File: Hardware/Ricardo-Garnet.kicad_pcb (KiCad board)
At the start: 4 copper layers, 38.5 x 90 mm, 193 parts, among them IC3 AP2205-W5-7, IC4 TPS61089RNRR, IC5 ADS131M04IRUKR, J1 RBUS, J2 USB_C_Receptacle_USB2.0, J3 Rotary Pot, J4 Conn_01x02_Male, J5 Conn_01x02_Male, J7 Conn_01x02_Male, J8 Conn_01x02_Male, J9 Conn_01x02_Male, P4 IN+, P5 IN-, P6 MOTOR1, P7 MOTOR2, P9 MOTOR3, Q1 IRFS7530, Q2 IRFS7530, Q3 IRFS7530, Q4 IRFS7530, Q5 IRFS7530, Q6 IRFS7530, U1 ESP32-S3, U10 MAX31856, U11 MAX31856, U3 DRV8302, U4 LM66200DRLR, U5 SC4215, U6 SN65HVD230, U7 MAX77827AEFD+T, U9 THVD2429, Y2 R940000171

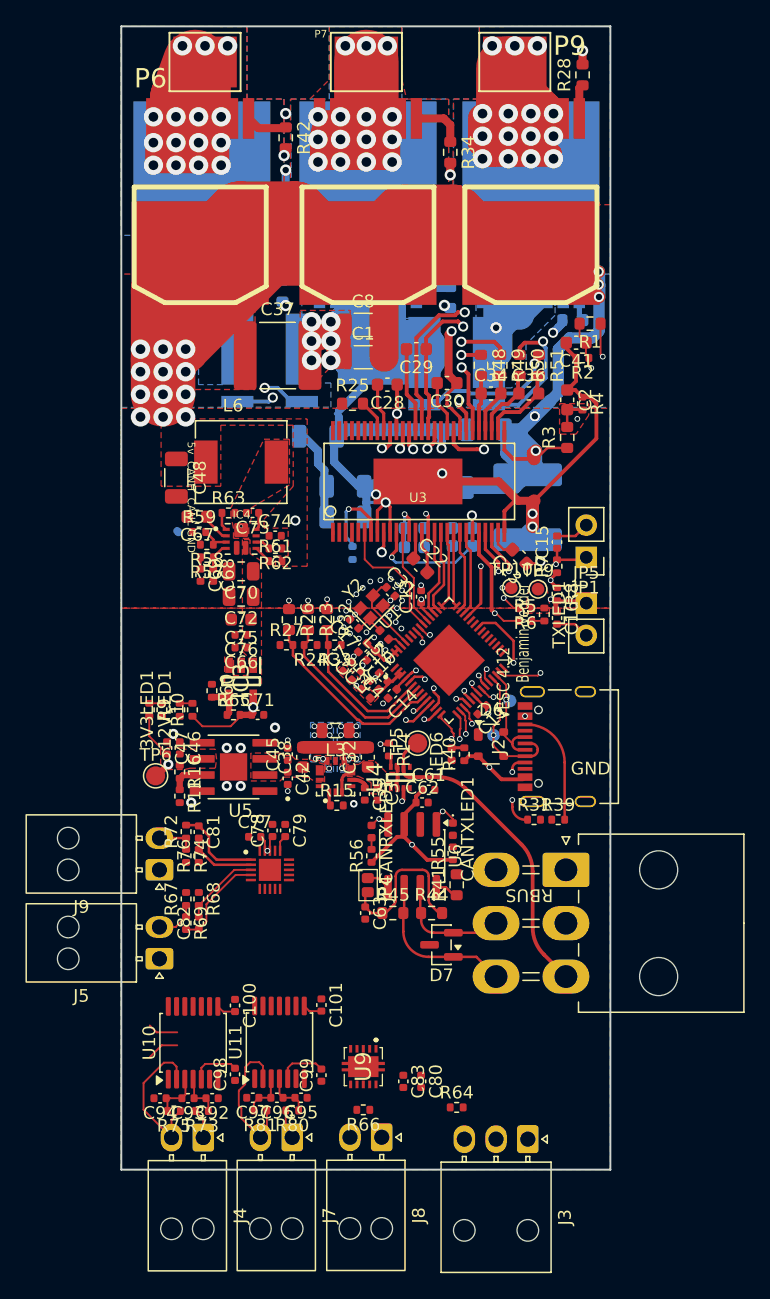
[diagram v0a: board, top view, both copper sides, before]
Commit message: close to 1st done
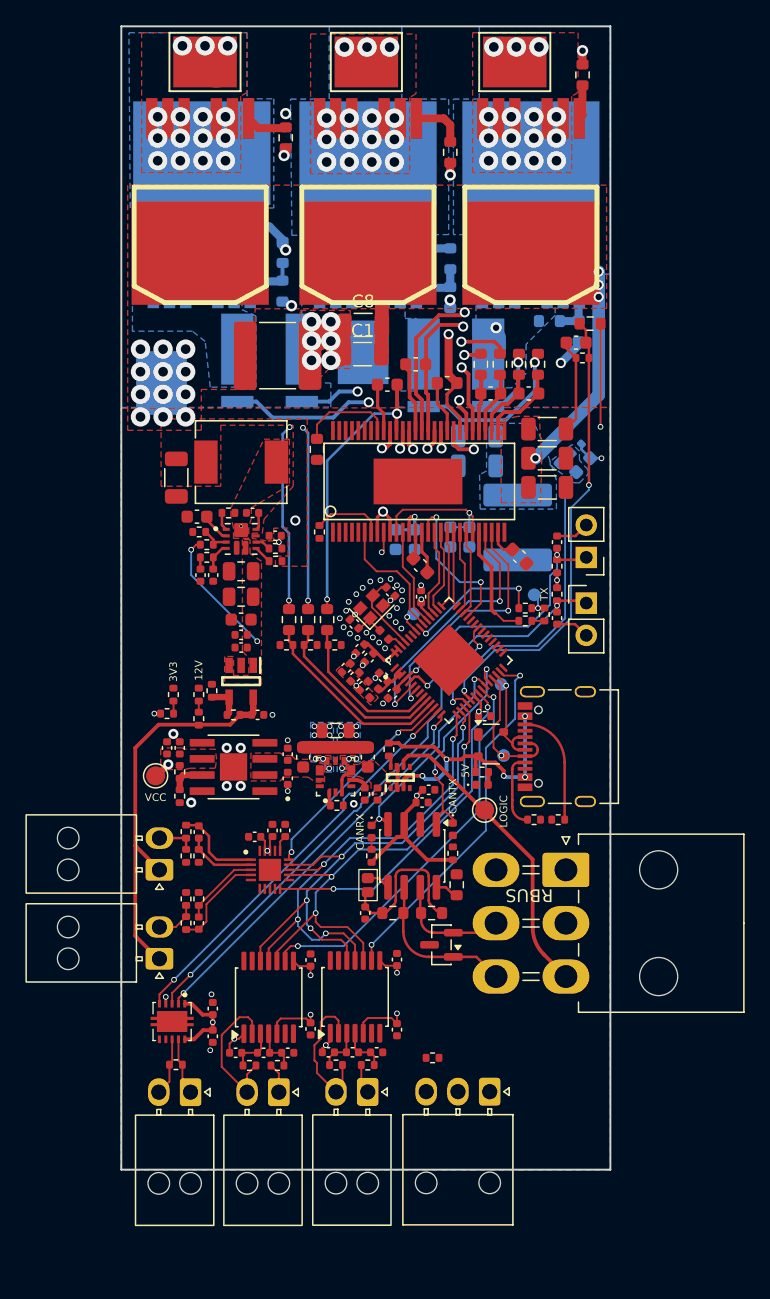
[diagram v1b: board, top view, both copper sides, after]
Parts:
- removed C34, C36: 2.2n, Capacitor_SMD:C_0603_1608Metric
- removed R48, R49, R50, R51: 100R, Resistor_SMD:R_0603_1608Metric
- added C19: 2.2n, Capacitor_SMD:C_0603_1608Metric, F.Cu at (107.6, 108.9)
- added C21: 2.2n, Capacitor_SMD:C_0603_1608Metric, F.Cu at (110.6, 108.9)
- added R12: 100R, Resistor_SMD:R_0603_1608Metric, F.Cu at (106.8, 106.6)
- added R13: 100R, Resistor_SMD:R_0603_1608Metric, F.Cu at (108.3, 106.6)
- added R17: 100R, Resistor_SMD:R_0603_1608Metric, F.Cu at (109.8, 106.6)
- added R18: 100R, Resistor_SMD:R_0603_1608Metric, F.Cu at (111.3, 106.6)
- C2, R3, R4: moved to B.Cu
- C43, C44, C49, R20: moved to F.Cu
- RXD: renamed from TP10; moved to B.Cu
- TXD: renamed from TP9; moved to B.Cu
- moved C43 18.1 mm to (112.0, 111.7)
- moved C80 17.4 mm to (85.7, 157.3)
- moved C49 16.1 mm to (112.0, 116.3)
- moved C44 16.0 mm to (112.0, 114.0)
- moved J8 15.5 mm to (84.0, 163.9)
- moved U9 15.5 mm to (82.5, 158.3)
- moved C83 15.4 mm to (85.7, 159.5)
- moved R66 15.2 mm to (82.8, 161.7)
- moved R30 10.5 mm to (112.2, 103.2), turned to 0 degrees
- moved RXD 7.97 mm to (101.5, 126.2), turned to 180 degrees
- moved LOGIC 7.45 mm to (107.1, 141.7)
- moved C96 6.94 mm to (96.7, 160.8)
- moved C97 6.94 mm to (94.8, 160.8)
- moved C98 6.94 mm to (93.4, 158.9)
- moved C99 6.94 mm to (100.2, 159.0)
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- renumbered 12VLED1 to 12V, 3V3LED1 to 3V3, CANRXLED1 to CANRX, CANTXLED1 to CANTX, TP2 to Dat+, TP1 to Dat-, TP5 to LOGIC, TXLED1 to TX, TP6 to VCC
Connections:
- net /Mosfet driver/H1_VS renamed /Mosfet driver/SH_A
- net /Mosfet driver/H2_VS renamed /Mosfet driver/SH_B
- net /Mosfet driver/H3_VS renamed /Mosfet driver/SH_C
- net /Mosfet driver/M_H1 renamed /Mosfet driver/GH_A
- net /Mosfet driver/M_H2 renamed /Mosfet driver/GH_B
- net /Mosfet driver/M_H3 renamed /Mosfet driver/GH_C
- net /Mosfet driver/M_L1 renamed /Mosfet driver/GL_A
- net /Mosfet driver/M_L2 renamed /Mosfet driver/GL_B
- net /Mosfet driver/M_L3 renamed /Mosfet driver/GL_C
- Q2 pad S: GND -> /Mosfet driver/SL_A
- Q6 pad S: GND -> /Mosfet driver/SL_C
- R30 pad 1: GND -> /Mosfet driver/SL_A
- R46 pad 1: GND -> /Mosfet driver/SL_C
- R53 pad 2: GND -> /Mosfet driver/SL_A
- R53 pad 3: /Mosfet driver/SH2_B -> Net-(R18-Pad1)
- R53 pad 4: /Mosfet driver/SH2_A -> Net-(R17-Pad1)
- R54 pad 1: GND -> /Mosfet driver/SL_C
- R54 pad 3: /Mosfet driver/SH1_A -> Net-(R12-Pad1)
- R54 pad 4: /Mosfet driver/SH1_B -> Net-(R13-Pad1)
- U1 pad 10: /BR_SO2 -> /SENS1
- U1 pad 11: /BR_SO1 -> /SENS2
- U1 pad 12: /AN_IN -> /ACD_CLK
- U1 pad 13: /MOS_TEMP -> /MOD_TX
- U1 pad 14: /HSPI_MISO -> /MOD_RX
- U1 pad 15: /HSPI_MOSI -> /HSPI_MISO
- U1 pad 16: /HSPI_SCLK -> /HSPI_MOSI
- U1 pad 17: /ACD_CLK -> /HSPI_SCLK
- U1 pad 18: /MOD_RX -> /AN_IN
- U1 pad 19: /MOD_TX -> /MOS_TEMP
- U1 pad 21: /TC_CS_0 -> /ACD_CS
- U1 pad 22: /TC_CS_1 -> /TC_CS_0
- U1 pad 27: /MOD_DE -> /TC_CS_1
- U1 pad 36: /ACD_CS -> /MOD_DE
- U1 pad 6: /SENS3 -> /BR_SO1
- U1 pad 7: /SENS1 -> /BR_SO2
- U1 pad 9: /SENS2 -> /SENS3
- U3 pad 30: Net-(U3-SP2) -> /Mosfet driver/SP2
- U3 pad 31: Net-(U3-SN2) -> /Mosfet driver/SN2
- U3 pad 32: Net-(U3-SP1) -> /Mosfet driver/SP1
- U3 pad 33: Net-(U3-SN1) -> /Mosfet driver/SN1
- U3 pad 34: GND -> /Mosfet driver/SL_C
- U3 pad 44: GND -> /Mosfet driver/SL_A
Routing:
- net V_SUPPLY: track 250.6 -> 60.7 mm, vias 17 -> 16
- net GND: track 256.9 -> 70.2 mm, vias 53 -> 54
- net VCC: track 157.8 -> 64.9 mm, vias 15 -> 17
- net /Mosfet driver/SH_B: track 171.3 -> 86.8 mm, vias 17 -> 18
- net /Mosfet driver/SH_A: track 160.4 -> 86.4 mm
- net /Mosfet driver/SH_C: track 157.0 -> 85.7 mm, vias 18 -> 19
- net /Mosfet driver/SL_C: track 0.00 -> 33.4 mm, vias 0 -> 2
- net /Mosfet driver/SL_A: track 0.00 -> 25.9 mm, vias 0 -> 2
- net Net-(R12-Pad1): track 0.00 -> 25.2 mm, vias 0 -> 2
- net /Mosfet driver/SH1_B: track 25.0 -> 0.00 mm, vias 2 -> 0
- net /Mosfet driver/SH1_A: track 24.0 -> 0.00 mm, vias 2 -> 0
- net Net-(R13-Pad1): track 0.00 -> 19.2 mm, vias 0 -> 2
- net /TC_CS_0: track 48.2 -> 31.2 mm, vias 1 -> 2
- net /MOD_TX: track 48.4 -> 32.4 mm, vias 1 -> 2
- net /MOD_RX: track 46.0 -> 31.3 mm, vias 1 -> 2
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- added copper zone on B.Cu, net /AN_IN
- added copper zone on B.Cu, net /Mosfet driver/SL_A
- added copper zone on B.Cu, net /Mosfet driver/SL_C
- added copper zone on In2.Cu, net VCC
- added copper zone on B.Cu, net V_SUPPLY
- removed copper zone on F.Cu, net /AN_IN
- removed copper zone on F.Cu, net /TXD
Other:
- board text added: "5V"
- board text removed: "3.3V"
- board text removed: "3.3v"
- board text removed: "5v"
- board text removed: "ADC"
- board text removed: "ADC2"
- board text removed: "Benjamin Vedder"
- board text removed: "CANH"
- board text removed: "CANL"
- board text removed: "CLK"
- board text removed: "DIO"
- board text removed: "GND"
- board text removed: "H1"
- board text removed: "H2"
- board text removed: "H3"
- board text removed: "MISO"
- board text removed: "MOSI"
- board text removed: "NSS"
- board text removed: "RST"
- board text removed: "RX"
- board text removed: "SCK"
- board text removed: "SCL"
- board text removed: "SDA"
- board text removed: "TEMP"
- board text removed: "TX"
- board text removed: "VESC 4.12"
- board text removed: "vedder.se"
